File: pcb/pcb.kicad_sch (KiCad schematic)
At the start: 28 parts, among them J1 USB_C_Receptacle_USB2.0_16P, SW1 SW_Push, U1 SRV05-4_C7420376, U2 XC6206P332MR, U3 STM32F072CBTx

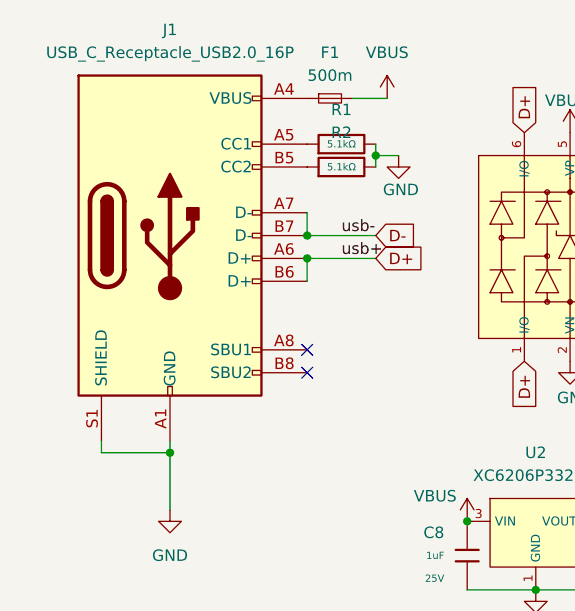
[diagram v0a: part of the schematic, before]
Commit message: jlcpcb USB-C
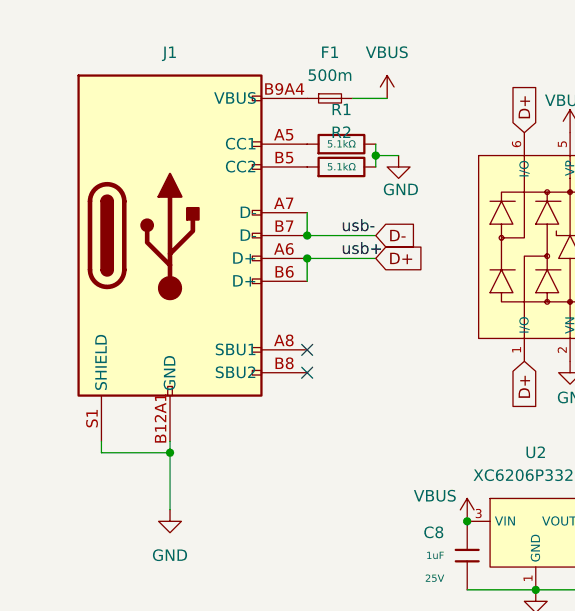
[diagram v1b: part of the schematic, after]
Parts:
- removed J1: USB_C_Receptacle_USB2.0_16P, PCM_marbastlib-various:USB_C_Receptacle_HRO_TYPE-C-31-M-12, symbol Connector:USB_C_Receptacle_USB2.0_16P
- added J1: Connector, USB-TYPE-C-16P, PCM_JLCPCB:TYPE-C-SMD_HX-TYPE-C-16PIN, symbol PCM_JLCPCB-Extended:Connector, USB-TYPE-C-16P
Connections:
- net D+: now also J1.A6 (D+), J1.B6 (D+)
- net D-: now also J1.A7 (D-), J1.B7 (D-)
- net GND: now also J1.A12B1 (GND), J1.B12A1 (GND), J1.S1 (SHIELD)
- net at R1.1: now also J1.A5 (CC1)
- net at R2.1: now also J1.B5 (CC2)
- net at F1.1: now also J1.A9B4 (VBUS), J1.B9A4 (VBUS)
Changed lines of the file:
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@@
 	)
 	(junction
+		(at 57.15 40.64)
+		(diameter 0)
+		(color 0 0 0 0)
+	)
+	(junction
 		(at 232.41 55.88)
 		(diameter 0)
@@
 	)
 	(junction
-		(at 57.15 40.64)
-		(diameter 0)
-		(color 0 0 0 0)
-	)
-	(junction
 		(at 57.15 43.18)
 		(diameter 0)
@@
 		(dnp no)
 		(fields_autoplaced yes)
-		(property "Reference" "#PWR04"
+		(property "Reference" "#PWR05"
 			(at 142.24 39.37 0)
 			(effects
@@
 			(project ""
 				(path "/c1d39311-56a5-4035-b0a7-7ad71eed89a6"
-					(reference "#PWR04")
+					(reference "#PWR05")
 					(unit 1)
 				)
@@
 		(on_board yes)
 		(dnp no)
-		(property "Reference" "#PWR06"
+		(property "Reference" "#PWR07"
 			(at 86.36 60.96 0)
 			(effects
@@
 			(project ""
 				(path "/c1d39311-56a5-4035-b0a7-7ad71eed89a6"
-					(reference "#PWR06")
+					(reference "#PWR07")
 					(unit 1)
 				)
@@
 		(dnp no)
 		(fields_autoplaced yes)
-		(property "Reference" "#PWR07"
+		(property "Reference" "#PWR06"
 			(at 196.85 52.07 0)
 			(effects
@@
 			(project ""
 				(path "/c1d39311-56a5-4035-b0a7-7ad71eed89a6"
-					(reference "#PWR07")
+					(reference "#PWR06")
 					(unit 1)
 				)
@@
 		(on_board yes)
 		(dnp no)
-		(property "Reference" "#PWR05"
+		(property "Reference" "#PWR02"
 			(at 86.36 33.02 0)
 			(effects
@@
 			(project ""
 				(path "/c1d39311-56a5-4035-b0a7-7ad71eed89a6"
-					(reference "#PWR05")
+					(reference "#PWR02")
 					(unit 1)
 				)
@@
 		(on_board yes)
 		(dnp no)
-		(property "Reference" "#PWR03"
+		(property "Reference" "#PWR04"
 			(at 124.46 36.83 0)
 			(effects
@@
 			(project ""
 				(path "/c1d39311-56a5-4035-b0a7-7ad71eed89a6"
-					(reference "#PWR03")
+					(reference "#PWR04")
 					(unit 1)
 				)
@@
 		(on_board yes)
 		(dnp no)
-		(property "Reference" "#PWR02"
+		(property "Reference" "#PWR03"
 			(at 67.31 38.1 0)
 			(effects
@@
 			(project ""
 				(path "/c1d39311-56a5-4035-b0a7-7ad71eed89a6"
-					(reference "#PWR02")
+					(reference "#PWR03")
 					(unit 1)
 				)
@@
 	)
 	(symbol
-		(lib_id "Connector:USB_C_Receptacle_USB2.0_16P")
-		(at 41.91 40.64 0)
-		(unit 1)
-		(exclude_from_sim no)
-		(in_bom yes)
-		(on_board yes)
-		(dnp no)
-		(fields_autoplaced yes)
-		(property "Reference" "J1"
-			(at 41.91 17.78 0)
-			(effects
-				(font
-					(size 1.27 1.27)
-				)
-			)
-		)
-		(property "Value" "USB_C_Receptacle_USB2.0_16P"
-			(at 41.91 20.32 0)
-			(effects
-				(font
-					(size 1.27 1.27)
-				)
-			)
-		)
-		(property "Footprint" "PCM_marbastlib-various:USB_C_Receptacle_HRO_TYPE-C-31-M-12"
-			(at 45.72 40.64 0)
-			(effects
-				(font
-					(size 1.27 1.27)
-				)
-				(hide yes)
-			)
-		)
-		(property "Datasheet" "https://www.usb.org/sites/default/files/documents/usb_type-c.zip"
-			(at 45.72 40.64 0)
-			(effects
-				(font
-					(size 1.27 1.27)
-				)
-				(hide yes)
-			)
-		)
-		(property "Description" "USB 2.0-only 16P Type-C Receptacle connector"
-			(at 41.91 40.64 0)
-			(effects
-				(font
-					(size 1.27 1.27)
-				)
-				(hide yes)
-			)
-		)
-		(pin "A6"
-		)
-		(pin "B7"
-		)
-		(pin "B4"
-		)
-		(pin "B6"
-		)
-		(pin "A5"
-		)
-		(pin "B9"
-		)
-		(pin "A7"
-		)
-		(pin "S1"
-		)
-		(pin "A9"
-		)
-		(pin "B12"
-		)
-		(pin "B1"
-		)
-		(pin "A12"
-		)
-		(pin "A1"
-		)
-		(pin "A4"
-		)
-		(pin "A8"
-		)
-		(pin "B5"
-		)
-		(pin "B8"
-		)
-		(instances
-			(project ""
-				(path "/c1d39311-56a5-4035-b0a7-7ad71eed89a6"
-					(reference "J1")
-					(unit 1)
-				)
-			)
-		)
-	)
-	(symbol
 		(lib_id "PCM_JLCPCB-Capacitors:0402,10uF")
 		(at 241.3 52.07 0)
@@
 					(unit 1)
 				)
+			)
+		)
+	)
+	(symbol
+		(lib_id "PCM_JLCPCB-Extended:Connector, USB-TYPE-C-16P")
+		(at 41.91 40.64 0)
+		(unit 1)
+		(exclude_from_sim no)
+		(in_bom yes)
+		(on_board yes)
+		(dnp no)
+		(fields_autoplaced yes)
+		(property "Reference" "J1"
+			(at 41.91 20.32 0)
+			(effects
+				(font
+					(size 1.27 1.27)
+				)
+			)
+		)
+		(property "Value" "Connector, USB-TYPE-C-16P"
+			(at 44.45 41.91 0)
+			(effects
+				(font
+					(size 1.27 1.27)
+				)
+				(hide yes)
+			)
+		)
+		(property "Footprint" "PCM_JLCPCB:TYPE-C-SMD_HX-TYPE-C-16PIN"
+			(at 41.91 50.8 0)
+			(effects
+				(font
+					(size 1.27 1.27)
+					(italic yes)
+				)
+				(hide yes)
+			)
+		)
+		(property "Datasheet" "https://atta.szlcsc.com/upload/public/pdf/source/20220920/0EF8F885FCCEA71F60E9E85152155021.pdf"
+			(at 39.624 40.513 0)
+			(effects
+				(font
+					(size 1.27 1.27)
+				)
+				(justify left)
+				(hide yes)
+			)
+		)
+		(property "Description" "3A 1 Horizontal attachment 16P Female -25℃~+85℃ Type-C SMD USB Connectors ROHS"
+			(at 44.45 39.37 0)
+			(effects
+				(font
+					(size 1.27 1.27)
+				)
+				(hide yes)
+			)
+		)
+		(property "LCSC" "C2927039"
+			(at 44.45 39.37 0)
+			(effects
+				(font
+					(size 1.27 1.27)
+				)
+				(hide yes)
+			)
+		)
+		(pin "B8"
+		)
+		(pin "A8"
+		)
+		(pin "A7"
+		)
+		(pin "B6"
+		)
+		(pin "A6"
+		)
+		(pin "B7"
+		)
+		(pin "S1"
+		)
+		(pin "B9A4"
+		)
+		(pin "A12B1"
+		)
+		(pin "B5"
+		)
+		(pin "B12A1"
+		)
+		(pin "A5"
+		)
+		(pin "A9B4"
+		)
+		(instances
+			(project ""
+				(path "/c1d39311-56a5-4035-b0a7-7ad71eed89a6"
+					(reference "J1")
+					(unit 1)
+				)
